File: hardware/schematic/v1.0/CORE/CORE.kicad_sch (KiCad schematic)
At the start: 82 parts, among them J1 Conn_01x06_Socket, J10 USB_C_Receptacle_USB2.0_16P, J11 Conn_01x06_Socket, J13 Conn_01x04_Socket, J14 Conn_01x03_Socket, J15 Conn_01x05_Socket, J16 Conn_01x04_Socket, J2 Conn_Coaxial, J26 Conn_01x04_Socket, J3 Conn_Coaxial, J4 Conn_Coaxial, J5 Conn_Coaxial, M1 ZYNQ7010&7020, U1 TXS02612RTWR, U10 IPEX1, U11 IPEX1, U2 TPS78633, U3 SD_Card, U4 IPEX1, U5 AMS1117-1.8, U6 CH340E, U7 FPC-6P, U8 IPEX1, U9 IPEX1

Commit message: sch update
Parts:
- removed BOOT_CFG1: CSW-2P, Counter:CSW DIP-2P, symbol Counter:CSW-2P
- removed C1, C11, C2, C3, C5, C6: 100nF, Capacitor_SMD:C_0402_1005Metric, symbol Device:C
- removed C12, C7: 10uF, Capacitor_SMD:C_0603_1608Metric, symbol Device:C
- removed C13: 1nF, Capacitor_SMD:C_0402_1005Metric, symbol Device:C
- removed C4: 10uF, Capacitor_SMD:C_0402_1005Metric, symbol Device:C
- removed D1, D2: AZ1143-04F.R7G, Counter:DFN2510P10E, symbol Counter:AZ1045-04F.R7G
- removed GE_PS1: HR911131A, Counter:HR911131A, symbol Counter:HR911131A_C
- removed J1, J11: Conn_01x06_Socket, Connector_PinHeader_2.54mm:PinHeader_1x06_P2.54mm_Vertical, symbol Connector:Conn_01x06_Socket
- removed J10: USB_C_Receptacle_USB2.0_16P, Connector_USB:USB_C_Receptacle_Palconn_UTC16-G, symbol Connector:USB_C_Receptacle_USB2.0_16P
- removed J14: Conn_01x03_Socket, Connector_PinHeader_2.54mm:PinHeader_1x03_P2.54mm_Vertical, symbol Connector:Conn_01x03_Socket
- removed J15: Conn_01x05_Socket, Connector_PinHeader_2.54mm:PinHeader_1x05_P2.54mm_Vertical, symbol Connector:Conn_01x05_Socket
- removed J2, J3, J4, J5: Conn_Coaxial, Connector_Coaxial:SMA_Amphenol_132289_EdgeMount, symbol Connector:Conn_Coaxial
- removed J26: Conn_01x04_Socket, Connector_PinHeader_2.54mm:PinHeader_1x04_P2.54mm_Vertical, symbol Connector:Conn_01x04_Socket
- removed JTAG1: JTAG, Counter:DC3_14P_2_7_DIP, symbol Counter:Header 7X2
- removed M1: ZYNQ7010&7020, Counter:ZYNQ7010&7020_CB, symbol Counter:ZYNQ7010&7020
- removed R1, R2, R3, R4: 33R, Resistor_SMD:R_0402_1005Metric, symbol Device:R
- removed R10, R9: 499R, Resistor_SMD:R_0402_1005Metric, symbol Device:R
- removed R11, R12: 20K, Resistor_SMD:R_0402_1005Metric, symbol Device:R
- removed R13, R14, R18: 10K, Resistor_SMD:R_0402_1005Metric, symbol Device:R
- removed R15, R19, R20, R21, R22, R23: 4.7K, Resistor_SMD:R_0402_1005Metric, symbol Device:R
- removed R16: 330, Resistor_SMD:R_0402_1005Metric, symbol Device:R
- removed R17, R38, R39: 0, Resistor_SMD:R_0402_1005Metric, symbol Device:R
- removed R36, R37: 5.1K, Resistor_SMD:R_0402_1005Metric, symbol Device:R
- removed R41, R42: 49.9, Resistor_SMD:R_0402_1005Metric, symbol Device:R
- removed RGB TFTLCD1: RGBLCD, AD:FPC-TOP40, symbol Counter:FPC-40
- removed U1: TXS02612RTWR, Counter:QFN24_RTW, symbol Counter:TXS02612RTWR
- removed U10, U11, U4, U8, U9: IPEX1, Counter:JLC_IPEX-1, symbol Counter:IPEX1
- removed U3: SD_Card, Counter:SIM-SMD_LX_XDFP-0090-012, symbol Counter:SD_Card
- removed U6: CH340E, Package_SO:MSOP-10_3x3mm_P0.5mm, symbol Interface_USB:CH340E
- removed U7: FPC-6P, symbol Counter:FPC-6P
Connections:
- no-connect marks 28 -> 0
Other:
- added sheet Comm_Periph (Comm_Periph.kicad_sch)
- added sheet Display (Display.kicad_sch)
- added sheet Signal (Signal.kicad_sch)
- added sheet Storage (Storage.kicad_sch)
- added sheet ZynqCore (ZynqCore.kicad_sch)
- note removed: "100 OHM TRACE"
- note removed: "50 OHM TRACE"
- note removed: "A20"
- note removed: "B13_L15_N"
- note removed: "B13_L15_P"
- note removed: "B13_L16_N"
- note removed: "B13_L16_P"
- note removed: "B13_L17_N"
- note removed: "B13_L17_P"
- note removed: "B13_L18_N"
- note removed: "B13_L18_P"
- note removed: "B13_L19_N"
- note removed: "B13_L19_P"
- note removed: "B13_L20_N"
- note removed: "B13_L20_P"
- note removed: "B13_L21_N"
- note removed: "B13_L21_P"
- note removed: "B13_L22_N"
- note removed: "B13_L22_P"
- note removed: "B13_L6N"
- note removed: "B19"
- note removed: "B20"
- note removed: "B34_IO0"
- note removed: "B34_IO25"
- note removed: "B34_L10_N"
- note removed: "B34_L10_P"
- note removed: "B34_L15_N"
- note removed: "B34_L15_P"
- note removed: "B34_L16_N"
- note removed: "B34_L16_P"
- note removed: "B34_L17_N"
- note removed: "B34_L17_P"
- note removed: "B34_L18_N"
- note removed: "B34_L18_P"
- note removed: "B34_L19_N"
- note removed: "B34_L19_P"
- note removed: "B34_L1_N"
- note removed: "B34_L1_P"
- note removed: "B34_L20_N"
- note removed: "B34_L20_P"
- note removed: "B34_L21_N"
- note removed: "B34_L21_P"
- note removed: "B34_L22_N"
- note removed: "B34_L22_P"
- note removed: "B34_L23_N"
- note removed: "B34_L23_P"
- note removed: "B34_L24_N"
- note removed: "B34_L24_P"
- note removed: "B34_L2_N"
- note removed: "B34_L2_P"
- note removed: "B34_L3_N"
- note removed: "B34_L3_P"
- note removed: "B34_L4_N"
- note removed: "B34_L4_P"
- note removed: "B34_L5_N"
- note removed: "B34_L5_P"
- note removed: "B34_L6_N"
- note removed: "B34_L6_P"
- note removed: "B34_L7_N"
- note removed: "B34_L7_P"
- note removed: "B34_L8_N"
- note removed: "B34_L8_P"
- note removed: "B34_L9_N"
- note removed: "B34_L9_P"
- note removed: "B35_IO0"
- note removed: "B35_IO25"
- note removed: "B35_L10_N"
- note removed: "B35_L10_P"
- note removed: "B35_L15_N"
- note removed: "B35_L15_P"
- note removed: "B35_L16_N"
- note removed: "B35_L16_P"
- note removed: "B35_L17_N"
- note removed: "B35_L17_P"
- note removed: "B35_L18_N"
- note removed: "B35_L18_P"
- note removed: "B35_L19_N"
- note removed: "B35_L19_P"
- note removed: "B35_L1_N"
- note removed: "B35_L1_P"
- note removed: "B35_L20_N"
- note removed: "B35_L20_P"
- note removed: "B35_L21_N"
- note removed: "B35_L21_P"
- note removed: "B35_L22_N"
- note removed: "B35_L22_P"
- note removed: "B35_L23_N"
- note removed: "B35_L23_P"
- note removed: "B35_L24_P"
- note removed: "B35_L2_N"
- note removed: "B35_L2_P"
- note removed: "B35_L3_N"
- note removed: "B35_L3_P"
- note removed: "B35_L4_N"
- note removed: "B35_L4_P"
- note removed: "B35_L5_N"
- note removed: "B35_L5_P"
- note removed: "B35_L6_N"
- note removed: "B35_L6_P"
- note removed: "B35_L7_N"
- note removed: "B35_L7_P"
- note removed: "B35_L8_N"
- note removed: "B35_L8_P"
- note removed: "B35_L9_N"
- note removed: "B35_L9_P"
- note removed: "C20"
- note removed: "D18"
- note removed: "D19"
- note removed: "D20"
- note removed: "E17"
- note removed: "E18"
- note removed: "E19"
- note removed: "ETHERNET(PS)"
- note removed: "F16"
- note removed: "F17"
- note removed: "F19"
- note removed: "F20"
- note removed: "G14"
- note removed: "G15"
- note removed: "G17"
- note removed: "G18"
- note removed: "G19"
- note removed: "G20"
- note removed: "H15"
- note removed: "H16"
- note removed: "H17"
- note removed: "H18"
- note removed: "H20"
- note removed: "J14"
- note removed: "J15"
- note removed: "J18"
- note removed: "J19"
- note removed: "J20"
- note removed: "JTAG"
- note removed: "K14"
- note removed: "K16"
- note removed: "K17"
- note removed: "K18"
- note removed: "K19"
- note removed: "L14"
- note removed: "L15"
- note removed: "L16"
- note removed: "L17"
- note removed: "L19"
- note removed: "L20"
- note removed: "M14"
- note removed: "M15"
- note removed: "M17"
- note removed: "M18"
- note removed: "M19"
- note removed: "M20"
- note removed: "MIO 4"
- note removed: "MIO 5"
- note removed: "MRCC B13_L12_N"
- note removed: "MRCC B13_L12_P"
- note removed: "MRCC B13_L13_N"
- note removed: "MRCC B13_L13_P"
- note removed: "MRCC B34_L12_N"
- note removed: "MRCC B34_L13_N"
- note removed: "MRCC B34_L13_P"
- note removed: "MRCC B35_L12_N"
- note removed: "MRCC B35_L12_P"
- note removed: "MRCC B35_L13_N"
- note removed: "MRCC B35_L13_P"
- note removed: "N15"
- note removed: "N16"
- note removed: "N17"
- note removed: "N18"
- note removed: "N20"
- note removed: "P14"
- note removed: "P15"
- note removed: "P16"
- note removed: "P18"
- note removed: "P19"
- note removed: "P20"
- note removed: "PS_MIO10"
- note removed: "PS_MIO11"
- note removed: "PS_MIO12"
- note removed: "PS_MIO13"
- note removed: "PS_MIO30"
- note removed: "PS_MIO31"
- note removed: "PS_MIO40"
- note removed: "PS_MIO41"
- note removed: "PS_MIO42"
- note removed: "PS_MIO43"
- note removed: "PS_MIO44"
- note removed: "PS_MIO45"
- note removed: "PS_MIO7"
- note removed: "PS_MIO8"
- note removed: "PS_MIO9"
- note removed: "R14"
- note removed: "R16"
- note removed: "R17"
- note removed: "R18"
- note removed: "R19"
- note removed: "RGB888"
- note removed: "SD_CARD"
- note removed: "SIGNAL"
- note removed: "SOCKET"
- note removed: "SRCC B13_L11_N"
- note removed: "SRCC B13_L11_P"
- note removed: "SRCC B13_L14_N"
- note removed: "SRCC B13_L14_P"
- note removed: "SRCC B34_L11_N"
- note removed: "SRCC B34_L11_P"
- note removed: "SRCC B34_L14_N"
- note removed: "SRCC B34_L14_P"
- note removed: "SRCC B35_L11_N"
- note removed: "SRCC B35_L11_P"
- note removed: "SRCC B35_L14_N"
- note removed: "SRCC B35_L14_P"
- note removed: "T10"
- note removed: "T11"
- note removed: "T12"
- note removed: "T14"
- note removed: "T15"
- note removed: "T16"
- note removed: "T17"
- note removed: "T19"
- note removed: "T20"
- note removed: "T5"
- note removed: "T9"
- note removed: "U10"
- note removed: "U12"
- note removed: "U13"
- note removed: "U14"
- note removed: "U15"
- note removed: "U17"
- note removed: "U19"
- note removed: "U20"
- note removed: "U5"
- note removed: "U7"
- note removed: "U8"
- note removed: "U9"
- note removed: "V10"
- note removed: "V11"
- note removed: "V12"
- note removed: "V13"
- note removed: "V15"
- note removed: "V16"
- note removed: "V17"
- note removed: "V18"
- note removed: "V20"
- note removed: "V5"
- note removed: "V6"
- note removed: "V7"
- note removed: "V8"
- note removed: "W10"
- note removed: "W11"
- note removed: "W13"
- note removed: "W14"
- note removed: "W15"
- note removed: "W16"
- note removed: "W18"
- note removed: "W19"
- note removed: "W20"
- note removed: "W6"
- note removed: "W8"
- note removed: "W9"
- note removed: "XADC"
- note removed: "Y11"
- note removed: "Y12"
- note removed: "Y13"
- note removed: "Y14"
- note removed: "Y16"
- note removed: "Y17"
- note removed: "Y18"
- note removed: "Y19"
- note removed: "Y6"
- note removed: "Y7"
- note removed: "Y8"
- note removed: "Y9"

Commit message: sch update
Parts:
- removed C10, C15, C17, C8: 10uF, Capacitor_SMD:C_0603_1608Metric, symbol Device:C
- removed C16, C18: 100nF, Capacitor_SMD:C_0603_1608Metric, symbol Device:C
- removed C19: 100nF, Capacitor_SMD:C_0402_1005Metric, symbol Device:C
- removed C9: 10nF, Capacitor_SMD:C_0402_1005Metric, symbol Device:C
- removed D3, D4, D5, D6: LED, LED_SMD:LED_0603_1608Metric, symbol Device:LED
- removed R40: 0, Resistor_SMD:R_0402_1005Metric, symbol Device:R
- removed R5, R6, R7, R8: 499R, Resistor_SMD:R_0402_1005Metric, symbol Device:R
- removed U2: TPS78633, Package_TO_SOT_SMD:SOT-223-6, symbol Counter:TPS78633
- removed U5: AMS1117-1.8, Package_TO_SOT_SMD:SOT-223-3_TabPin2, symbol Regulator_Linear:AMS1117-1.8
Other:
- added sheet Power (Power.kicad_sch)
- note removed: "POWER"
- note removed: "PS/PL LED"
- moved on the sheet: J13, J16

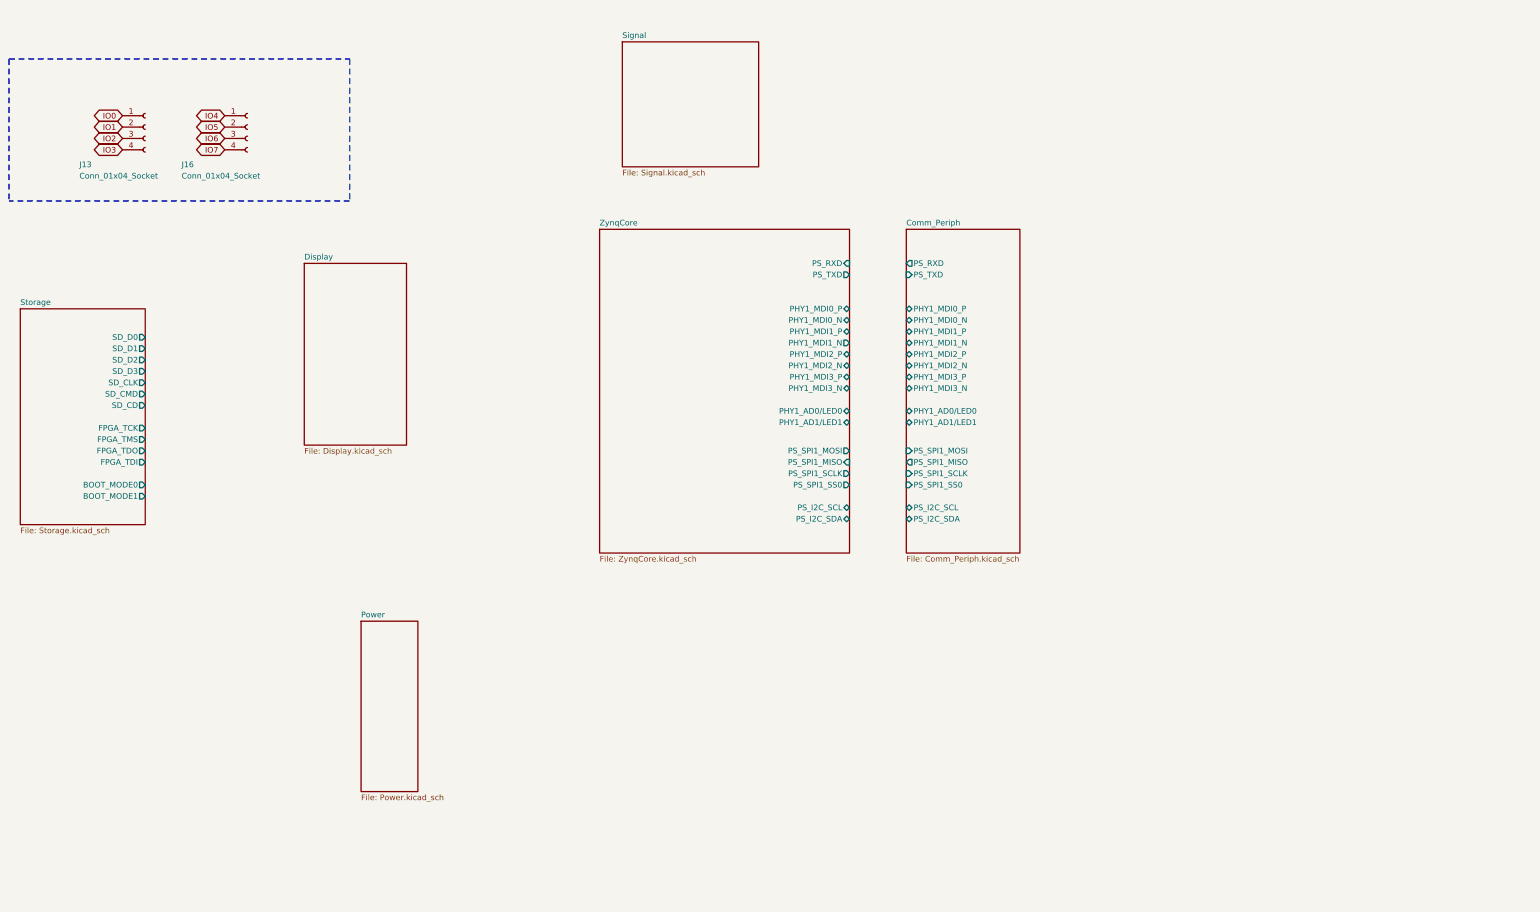
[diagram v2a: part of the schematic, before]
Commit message: sch update
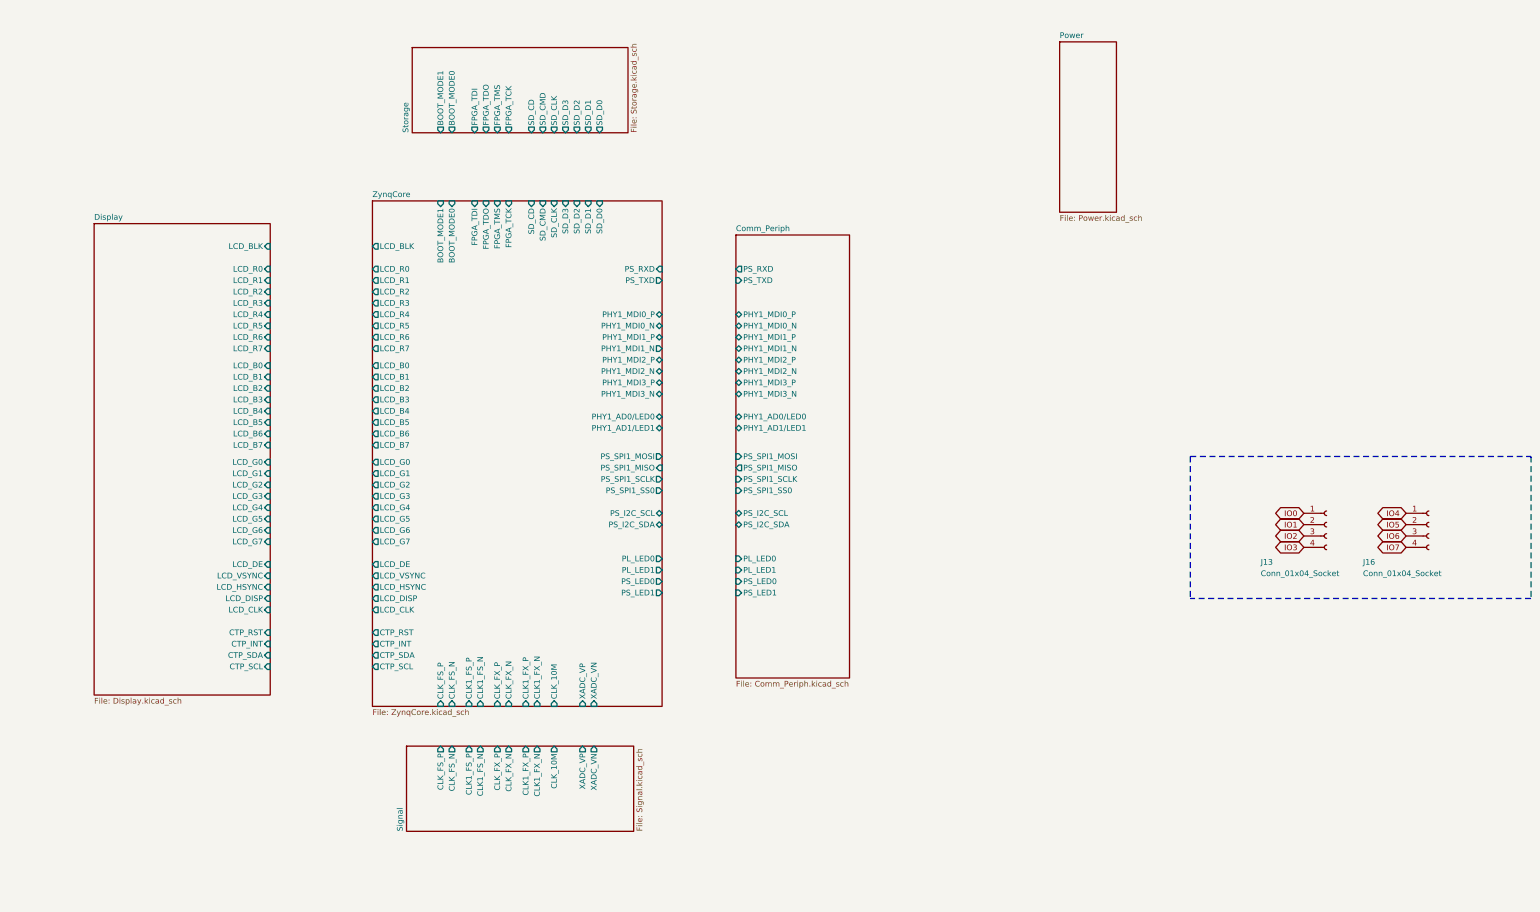
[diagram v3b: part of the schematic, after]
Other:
- sheet Comm_Periph ports: added PL_LED0, PL_LED1, PS_LED0, PS_LED1; removed none
- sheet Display ports: added CTP_INT, CTP_RST, CTP_SCL, CTP_SDA, LCD_B0, LCD_B1, LCD_B2, LCD_B3, LCD_B4, LCD_B5, LCD_B6, LCD_B7, LCD_BLK, LCD_CLK, LCD_DE, LCD_DISP, LCD_G0, LCD_G1, LCD_G2, LCD_G3, LCD_G4, LCD_G5, LCD_G6, LCD_G7, LCD_HSYNC, LCD_R0, LCD_R1, LCD_R2, LCD_R3, LCD_R4, LCD_R5, LCD_R6, LCD_R7, LCD_VSYNC; removed none
- sheet Signal ports: added CLK1_FS_N, CLK1_FS_P, CLK1_FX_N, CLK1_FX_P, CLK_10M, CLK_FS_N, CLK_FS_P, CLK_FX_N, CLK_FX_P, XADC_VN, XADC_VP; removed none
- sheet ZynqCore ports: added BOOT_MODE0, BOOT_MODE1, CLK1_FS_N, CLK1_FS_P, CLK1_FX_N, CLK1_FX_P, CLK_10M, CLK_FS_N, CLK_FS_P, CLK_FX_N, CLK_FX_P, CTP_INT, CTP_RST, CTP_SCL, CTP_SDA, FPGA_TCK, FPGA_TDI, FPGA_TDO, FPGA_TMS, LCD_B0, LCD_B1, LCD_B2, LCD_B3, LCD_B4, LCD_B5, LCD_B6, LCD_B7, LCD_BLK, LCD_CLK, LCD_DE, LCD_DISP, LCD_G0, LCD_G1, LCD_G2, LCD_G3, LCD_G4, LCD_G5, LCD_G6, LCD_G7, LCD_HSYNC, LCD_R0, LCD_R1, LCD_R2, LCD_R3, LCD_R4, LCD_R5, LCD_R6, LCD_R7, LCD_VSYNC, PL_LED0, PL_LED1, PS_LED0, PS_LED1, SD_CD, SD_CLK, SD_CMD, SD_D0, SD_D1, SD_D2, SD_D3, XADC_VN, XADC_VP; removed none
- moved on the sheet: J13, J16

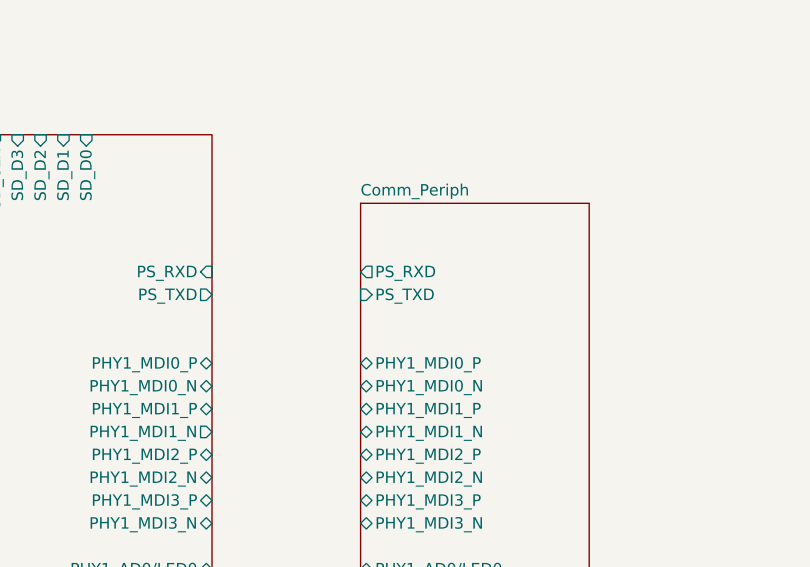
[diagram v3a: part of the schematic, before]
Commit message: sch update
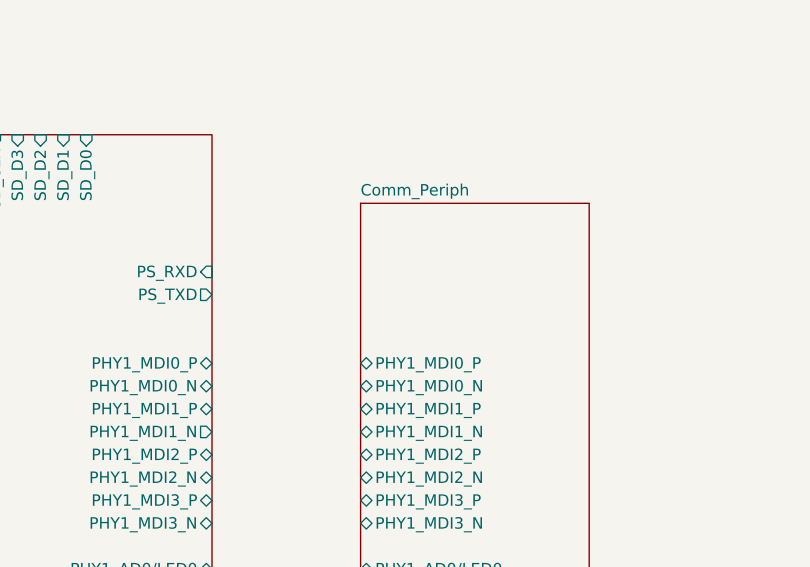
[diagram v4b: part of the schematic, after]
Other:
- sheet Comm_Periph ports: added none; removed PS_RXD, PS_TXD
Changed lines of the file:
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@@
-			)
-		)
-		(pin "PS_RXD" output
-			(at 189.23 68.58 180)
-			(effects
-				(font
-					(size 1.27 1.27)
-				)
-				(justify left)
-			)
-		)
-		(pin "PS_TXD" input
-			(at 189.23 71.12 180)
-			(effects
-				(font
-					(size 1.27 1.27)
-				)
-				(justify left)
 			)
 		)
